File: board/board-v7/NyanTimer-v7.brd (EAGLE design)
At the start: 136 x 45 mm, 51 parts, among them IC1 7815DT, IC2 MAX232, IC3 7815DT, SW1 AKIZUKI_SWITCH, U1 328P

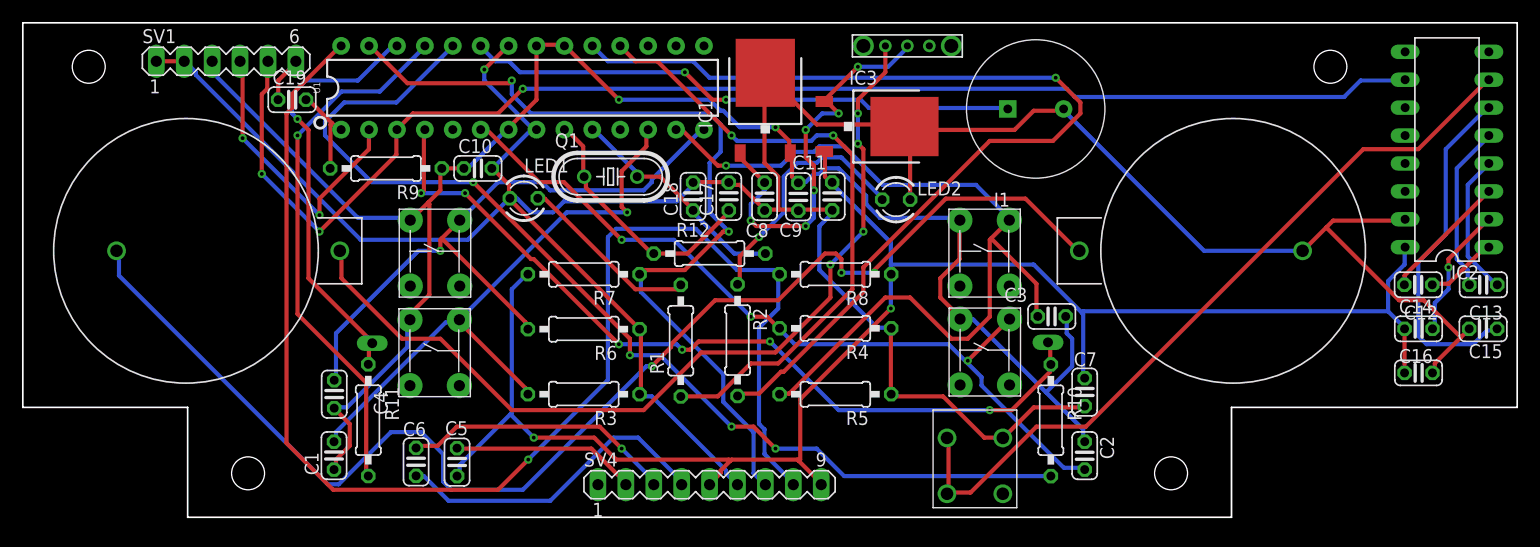
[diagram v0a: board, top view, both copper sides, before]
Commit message: changed pad
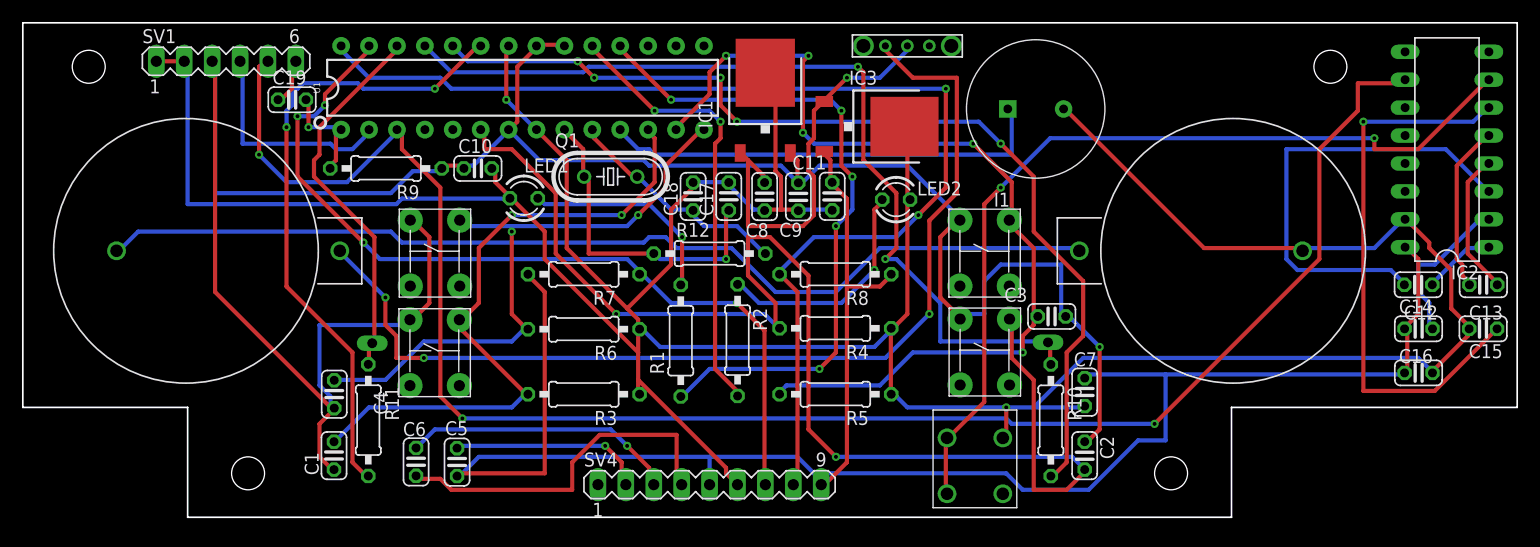
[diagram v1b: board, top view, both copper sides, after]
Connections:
- net BUZ+: now also U1.11; no longer U1.23
- net PADLIN: now also U1.23; no longer U1.25
- net PADR: now also U1.25; no longer U1.4
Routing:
- net +5V: track 160.4 -> 214.8 mm, vias 2 -> 1
- net LEDG: track 90.7 -> 40.6 mm, vias 1 -> 2
- net GND: track 278.8 -> 323.7 mm, vias 1 -> 2
- net SW2: track 73.8 -> 117.9 mm, vias 3 -> 2
- net T2IN: track 124.4 -> 159.8 mm
- net N$9: track 11.7 -> 41.7 mm
- net VCC: track 155.5 -> 185.4 mm, vias 2 -> 0
- net N$7: track 118.8 -> 92.8 mm, vias 3 -> 0
- net SCL: track 125.4 -> 104.5 mm, vias 1 -> 2
- net N$14: track 31.6 -> 50.9 mm, vias 0 -> 1
- net VSW: track 81.8 -> 92.5 mm, vias 4 -> 3
- net PHONE: track 69.9 -> 79.8 mm, vias 0 -> 2
- net BUZ+: track 50.4 -> 41.0 mm, vias 2 -> 0
- net PADLIN: track 48.6 -> 57.9 mm, vias 1 -> 2
- net SW3: track 78.8 -> 85.3 mm, vias 1 -> 5
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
